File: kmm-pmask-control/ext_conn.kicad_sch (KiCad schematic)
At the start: 14 parts, among them J1 F31L-1A7H1-11030, U1 PCA9517ADP

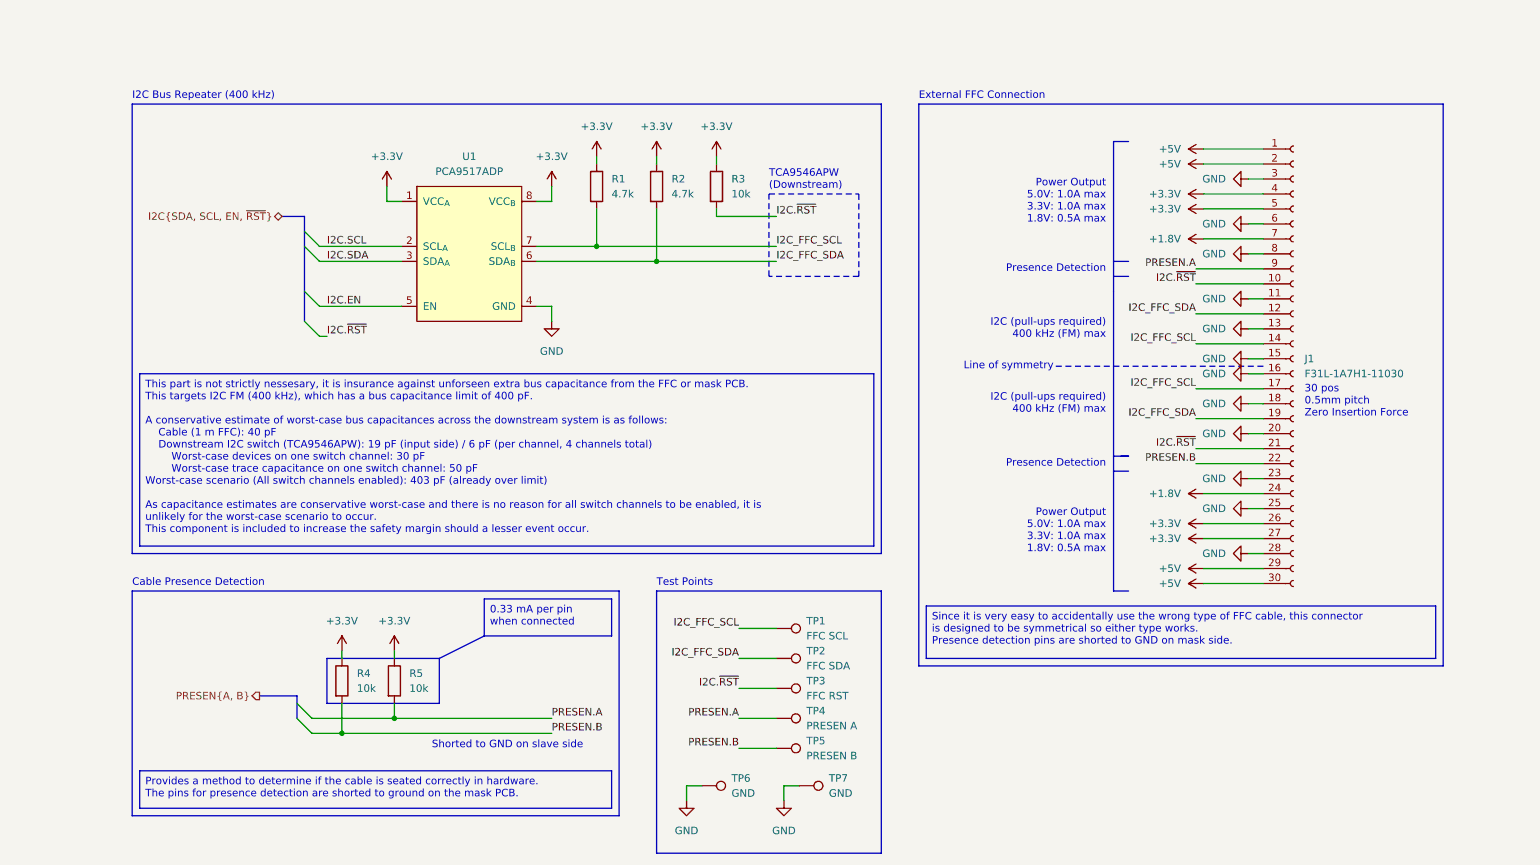
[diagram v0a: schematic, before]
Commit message: Initial draft of control board
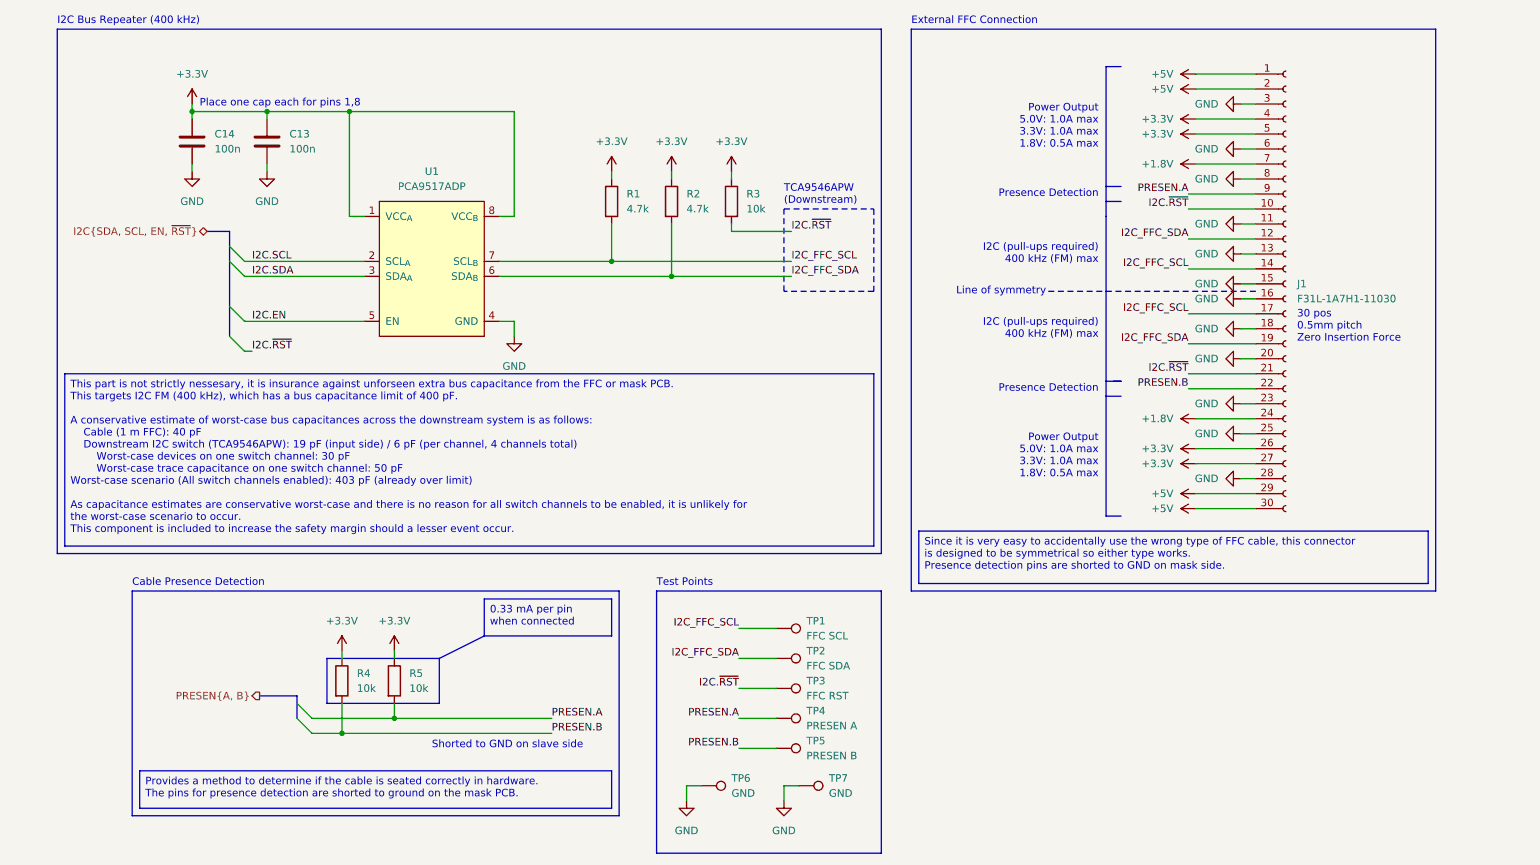
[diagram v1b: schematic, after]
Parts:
- added C13, C14: 100n, Capacitor_SMD:C_0402_1005Metric_Pad0.74x0.62mm_HandSolder, symbol Device:C
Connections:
- net +3.3V: now also C13.1, C14.1
- net GND: now also C13.2, C14.2
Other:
- note added: "Place one cap each for pins 1,8"
- moved on the sheet: J1, R1, R2, R3, U1

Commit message: Initial PCB Layout
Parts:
- TP1, TP2, TP3, TP4, TP5, TP6, TP7: footprint TestPoint:TestPoint_Pad_D1.5mm -> TestPoint:TestPoint_Pad_D1.0mm
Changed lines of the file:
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@@
 			)
 		)
-		(property "Footprint" "TestPoint:TestPoint_Pad_D1.5mm"
+		(property "Footprint" "TestPoint:TestPoint_Pad_D1.0mm"
 			(at 147.32 132.08 0)
 			(hide yes)
@@
 			)
 		)
-		(property "Footprint" "TestPoint:TestPoint_Pad_D1.5mm"
+		(property "Footprint" "TestPoint:TestPoint_Pad_D1.0mm"
 			(at 134.62 158.75 0)
 			(hide yes)
@@
 			)
 		)
-		(property "Footprint" "TestPoint:TestPoint_Pad_D1.5mm"
+		(property "Footprint" "TestPoint:TestPoint_Pad_D1.0mm"
 			(at 147.32 152.4 0)
 			(hide yes)
@@
 			)
 		)
-		(property "Footprint" "TestPoint:TestPoint_Pad_D1.5mm"
+		(property "Footprint" "TestPoint:TestPoint_Pad_D1.0mm"
 			(at 151.13 158.75 0)
 			(hide yes)
@@
 			)
 		)
-		(property "Footprint" "TestPoint:TestPoint_Pad_D1.5mm"
+		(property "Footprint" "TestPoint:TestPoint_Pad_D1.0mm"
 			(at 147.32 137.16 0)
 			(hide yes)
@@
 			)
 		)
-		(property "Footprint" "TestPoint:TestPoint_Pad_D1.5mm"
+		(property "Footprint" "TestPoint:TestPoint_Pad_D1.0mm"
 			(at 147.32 142.24 0)
 			(hide yes)
@@
 			)
 		)
-		(property "Footprint" "TestPoint:TestPoint_Pad_D1.5mm"
+		(property "Footprint" "TestPoint:TestPoint_Pad_D1.0mm"
 			(at 147.32 147.32 0)
 			(hide yes)
